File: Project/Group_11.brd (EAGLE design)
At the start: 29 parts, among them J1 POWER_JACKPTH_LOCK, U1 +12v

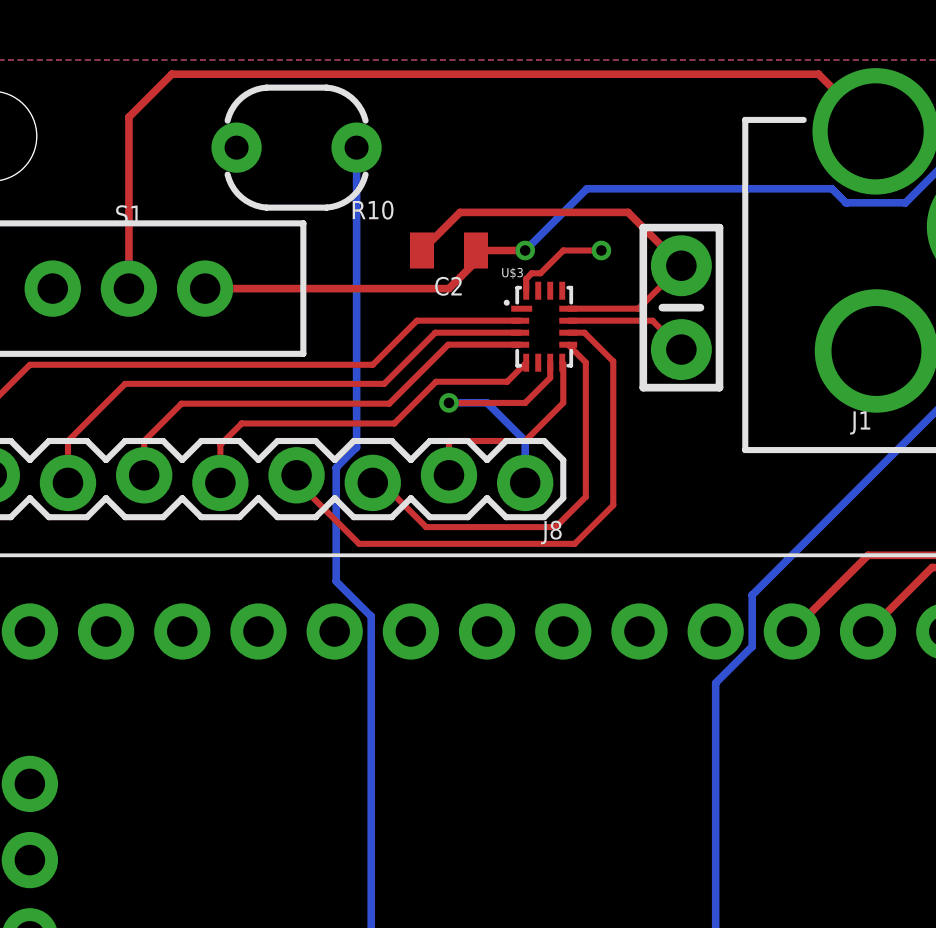
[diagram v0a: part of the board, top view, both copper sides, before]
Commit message: Aggiunta collegamenti board
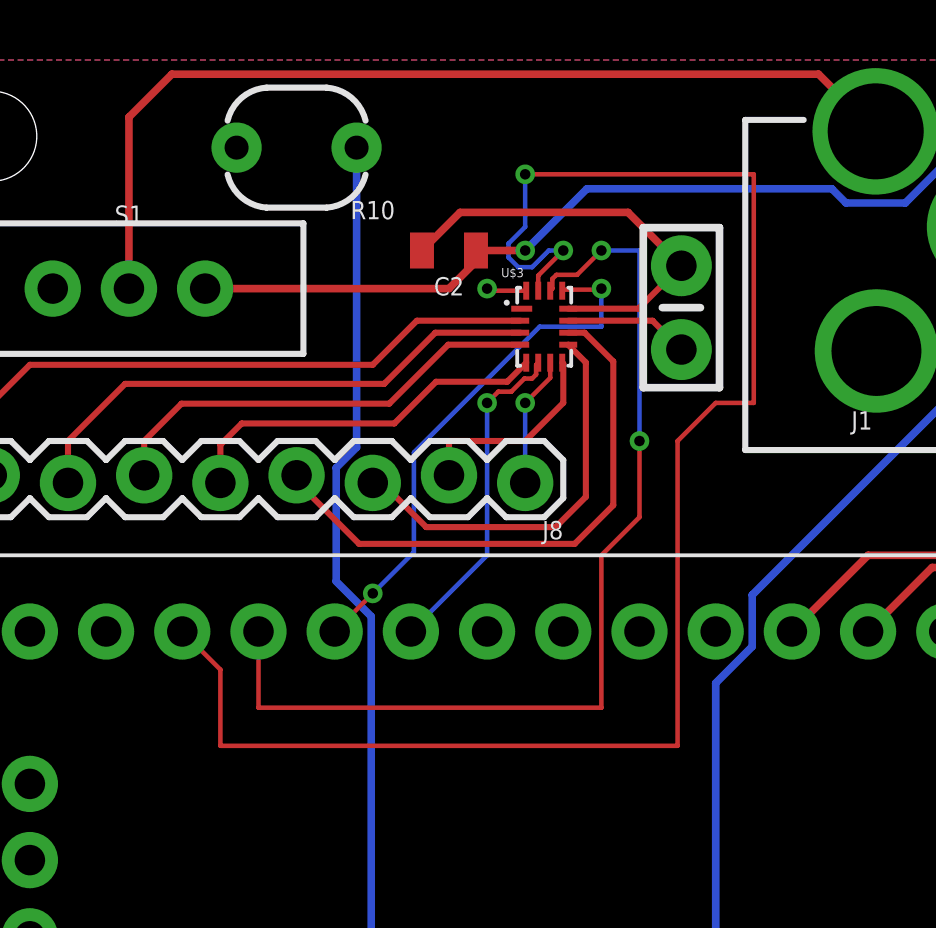
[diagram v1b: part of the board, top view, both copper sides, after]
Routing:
- net MUX_A0: track 0.00 -> 54.9 mm, vias 0 -> 2
- net MUX_A1: track 0.00 -> 33.5 mm, vias 0 -> 2
- net MUX_A2: track 0.00 -> 17.7 mm, vias 0 -> 2
- net MUX_OUT: track 0.00 -> 11.1 mm, vias 0 -> 1
- net N$11: track 8.69 -> 4.35 mm
- net 5V: track 46.6 -> 44.7 mm
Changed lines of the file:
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@@
 <wire x1="21.755" y1="38.3" x2="24.56501875" y2="38.3" width="0.2032" layer="1"/>
 <wire x1="24.56501875" y1="38.3" x2="25.527" y2="37.338" width="0.2032" layer="1"/>
-<wire x1="20.53926875" y1="39.8794" x2="20.8294" y2="39.8794" width="0.2032" layer="1"/>
-<wire x1="20.8294" y1="39.8794" x2="21.59" y2="40.64" width="0.2032" layer="1"/>
-<wire x1="21.59" y1="40.64" x2="22.86" y2="40.64" width="0.2032" layer="1"/>
-<via x="22.86" y="40.64" extent="1-16" drill="0.35"/>
+<via x="19.05" y="39.37" extent="1-16" drill="0.35"/>
 <wire x1="41.314" y1="33.147" x2="41.06" y2="32.893" width="0.254" layer="1"/>
 <wire x1="41.06" y1="32.893" x2="38.1" y2="32.893" width="0.254" layer="1"/>
@@
 <vertex x="0.508" y="1.27"/>
 </polygon>
-<wire x1="20.355" y1="39.3" x2="20.355" y2="39.69513125" width="0.2032" layer="1"/>
-<wire x1="20.355" y1="39.69513125" x2="20.53926875" y2="39.8794" width="0.2032" layer="1"/>
 <wire x1="41.91" y1="34.837" x2="40.386" y2="36.361" width="0.254" layer="1"/>
 <wire x1="40.386" y1="36.361" x2="40.386" y2="38.139" width="0.254" layer="1"/>
 <wire x1="41.314" y1="33.147" x2="41.314" y2="34.241" width="0.254" layer="1"/>
 <wire x1="41.314" y1="34.241" x2="41.91" y2="34.837" width="0.254" layer="1"/>
+<wire x1="20.355" y1="39.3" x2="19.12" y2="39.3" width="0.1524" layer="1"/>
+<wire x1="19.12" y1="39.3" x2="19.05" y2="39.37" width="0.1524" layer="1"/>
 </signal>
 <signal name="N$9">
@@
 <contactref element="J8" pad="1"/>
 <contactref element="U$3" pad="7"/>
-<wire x1="20.32" y1="35.56" x2="17.78" y2="35.56" width="0.2032" layer="1"/>
-<via x="17.78" y="35.56" extent="1-16" drill="0.35"/>
-<wire x1="17.78" y1="35.56" x2="19.05" y2="35.56" width="0.254" layer="16"/>
-<wire x1="19.05" y1="35.56" x2="20.32" y2="34.29" width="0.254" layer="16"/>
-<wire x1="20.32" y1="34.29" x2="20.32" y2="32.893" width="0.254" layer="16"/>
-<wire x1="21.155" y1="36.9" x2="21.155" y2="36.395" width="0.2032" layer="1"/>
-<wire x1="21.155" y1="36.395" x2="20.32" y2="35.56" width="0.2032" layer="1"/>
+<wire x1="20.32" y1="32.893" x2="20.32" y2="35.56" width="0.1524" layer="16"/>
+<via x="20.32" y="35.56" extent="1-16" drill="0.35"/>
+<wire x1="20.32" y1="35.56" x2="21.155" y2="36.395" width="0.1524" layer="1"/>
+<wire x1="21.155" y1="36.395" x2="21.155" y2="36.9" width="0.1524" layer="1"/>
 </signal>
 <signal name="N$12">
@@
 <contactref element="U$3" pad="6"/>
 <contactref element="U$2" pad="21"/>
-<wire x1="16.51" y1="27.94" x2="20.755" y2="36.9" width="0" layer="19" extent="1-1"/>
+<wire x1="16.51" y1="27.94" x2="19.05" y2="30.48" width="0.1524" layer="16"/>
+<wire x1="19.05" y1="30.48" x2="19.05" y2="35.56" width="0.1524" layer="16"/>
+<via x="19.05" y="35.56" extent="1-16" drill="0.35"/>
+<wire x1="19.05" y1="35.56" x2="19.4248" y2="35.9348" width="0.1524" layer="1"/>
+<wire x1="19.4248" y1="35.9348" x2="19.856775" y2="35.9348" width="0.1524" layer="1"/>
+<wire x1="20.293375" y1="36.3714" x2="20.5496875" y2="36.3714" width="0.1524" layer="1"/>
+<wire x1="19.856775" y1="35.9348" x2="20.293375" y2="36.3714" width="0.1524" layer="1"/>
+<wire x1="20.6852" y1="36.8302" x2="20.755" y2="36.9" width="0.1524" layer="1"/>
+<wire x1="20.5496875" y1="36.3714" x2="20.6852" y2="36.5069125" width="0.1524" layer="1"/>
+<wire x1="20.6852" y1="36.5069125" x2="20.6852" y2="36.8302" width="0.1524" layer="1"/>
 </signal>
 <signal name="MUX_A0">
 <contactref element="U$3" pad="15"/>
 <contactref element="U$2" pad="24"/>
-<wire x1="8.89" y1="27.94" x2="20.755" y2="39.3" width="0" layer="19" extent="1-1"/>
+<wire x1="8.89" y1="27.94" x2="10.16" y2="26.67" width="0.1524" layer="1"/>
+<wire x1="10.16" y1="26.67" x2="10.16" y2="24.13" width="0.1524" layer="1"/>
+<wire x1="10.16" y1="24.13" x2="25.4" y2="24.13" width="0.1524" layer="1"/>
+<wire x1="25.4" y1="24.13" x2="25.4" y2="34.29" width="0.1524" layer="1"/>
+<wire x1="25.4" y1="34.29" x2="26.67" y2="35.56" width="0.1524" layer="1"/>
+<wire x1="26.67" y1="35.56" x2="27.94" y2="35.56" width="0.1524" layer="1"/>
+<wire x1="27.94" y1="35.56" x2="27.94" y2="43.18" width="0.1524" layer="1"/>
+<wire x1="27.94" y1="43.18" x2="20.32" y2="43.18" width="0.1524" layer="1"/>
+<via x="20.32" y="43.18" extent="1-16" drill="0.35"/>
+<wire x1="19.764" y1="40.87030625" x2="19.764" y2="40.40969375" width="0.1524" layer="16"/>
+<wire x1="19.764" y1="40.40969375" x2="20.08969375" y2="40.084" width="0.1524" layer="16"/>
+<wire x1="20.08969375" y1="40.084" x2="20.55030625" y2="40.084" width="0.1524" layer="16"/>
+<wire x1="20.32" y1="43.18" x2="20.32" y2="41.42630625" width="0.1524" layer="16"/>
+<wire x1="20.32" y1="41.42630625" x2="19.764" y2="40.87030625" width="0.1524" layer="16"/>
+<wire x1="20.55030625" y1="40.084" x2="21.10630625" y2="40.64" width="0.1524" layer="16"/>
+<wire x1="21.10630625" y1="40.64" x2="21.59" y2="40.64" width="0.1524" layer="16"/>
+<via x="21.59" y="40.64" extent="1-16" drill="0.35"/>
+<wire x1="21.59" y1="40.64" x2="20.755" y2="39.805" width="0.1524" layer="1"/>
+<wire x1="20.755" y1="39.805" x2="20.755" y2="39.3" width="0.1524" layer="1"/>
 </signal>
 <signal name="MUX_A1">
 <contactref element="U$3" pad="14"/>
 <contactref element="U$2" pad="23"/>
-<wire x1="11.43" y1="27.94" x2="21.155" y2="39.3" width="0" layer="19" extent="1-1"/>
+<wire x1="11.43" y1="27.94" x2="11.43" y2="25.4" width="0.1524" layer="1"/>
+<wire x1="11.43" y1="25.4" x2="22.86" y2="25.4" width="0.1524" layer="1"/>
+<wire x1="22.86" y1="25.4" x2="22.86" y2="30.48" width="0.1524" layer="1"/>
+<wire x1="22.86" y1="30.48" x2="24.13" y2="31.75" width="0.1524" layer="1"/>
+<wire x1="24.13" y1="31.75" x2="24.13" y2="34.29" width="0.1524" layer="1"/>
+<via x="24.13" y="34.29" extent="1-16" drill="0.35"/>
+<wire x1="24.13" y1="34.29" x2="24.13" y2="40.64" width="0.1524" layer="16"/>
+<wire x1="24.13" y1="40.64" x2="22.86" y2="40.64" width="0.1524" layer="16"/>
+<via x="22.86" y="40.64" extent="1-16" drill="0.35"/>
+<wire x1="21.3603125" y1="39.8286" x2="21.2264" y2="39.6946875" width="0.1524" layer="1"/>
+<wire x1="22.86" y1="40.64" x2="22.0486" y2="39.8286" width="0.1524" layer="1"/>
+<wire x1="21.2264" y1="39.6946875" x2="21.2264" y2="39.3714" width="0.1524" layer="1"/>
+<wire x1="21.2264" y1="39.3714" x2="21.155" y2="39.3" width="0.1524" layer="1"/>
+<wire x1="22.0486" y1="39.8286" x2="21.3603125" y2="39.8286" width="0.1524" layer="1"/>
 </signal>
 <signal name="MUX_A2">
 <contactref element="U$3" pad="13"/>
 <contactref element="U$2" pad="22"/>
-<wire x1="13.97" y1="27.94" x2="21.555" y2="39.3" width="0" layer="19" extent="1-1"/>
+<wire x1="13.97" y1="27.94" x2="15.24" y2="29.21" width="0.1524" layer="1"/>
+<via x="15.24" y="29.21" extent="1-16" drill="0.35"/>
+<wire x1="15.24" y1="29.21" x2="16.6116" y2="30.5816" width="0.1524" layer="16"/>
+<wire x1="16.6116" y1="30.5816" x2="16.6116" y2="33.90790625" width="0.1524" layer="16"/>
+<wire x1="21.555" y1="39.335" x2="21.555" y2="39.3" width="0.1524" layer="1"/>
+<wire x1="16.6116" y1="33.90790625" x2="20.80369375" y2="38.1" width="0.1524" layer="16"/>
+<wire x1="20.80369375" y1="38.1" x2="22.86" y2="38.1" width="0.1524" layer="16"/>
+<wire x1="22.86" y1="38.1" x2="22.86" y2="39.37" width="0.1524" layer="16"/>
+<via x="22.86" y="39.37" extent="1-16" drill="0.35"/>
+<wire x1="22.86" y1="39.37" x2="22.825" y2="39.335" width="0.1524" layer="1"/>
+<wire x1="22.825" y1="39.335" x2="21.555" y2="39.335" width="0.1524" layer="1"/>
 </signal>
 </signals>

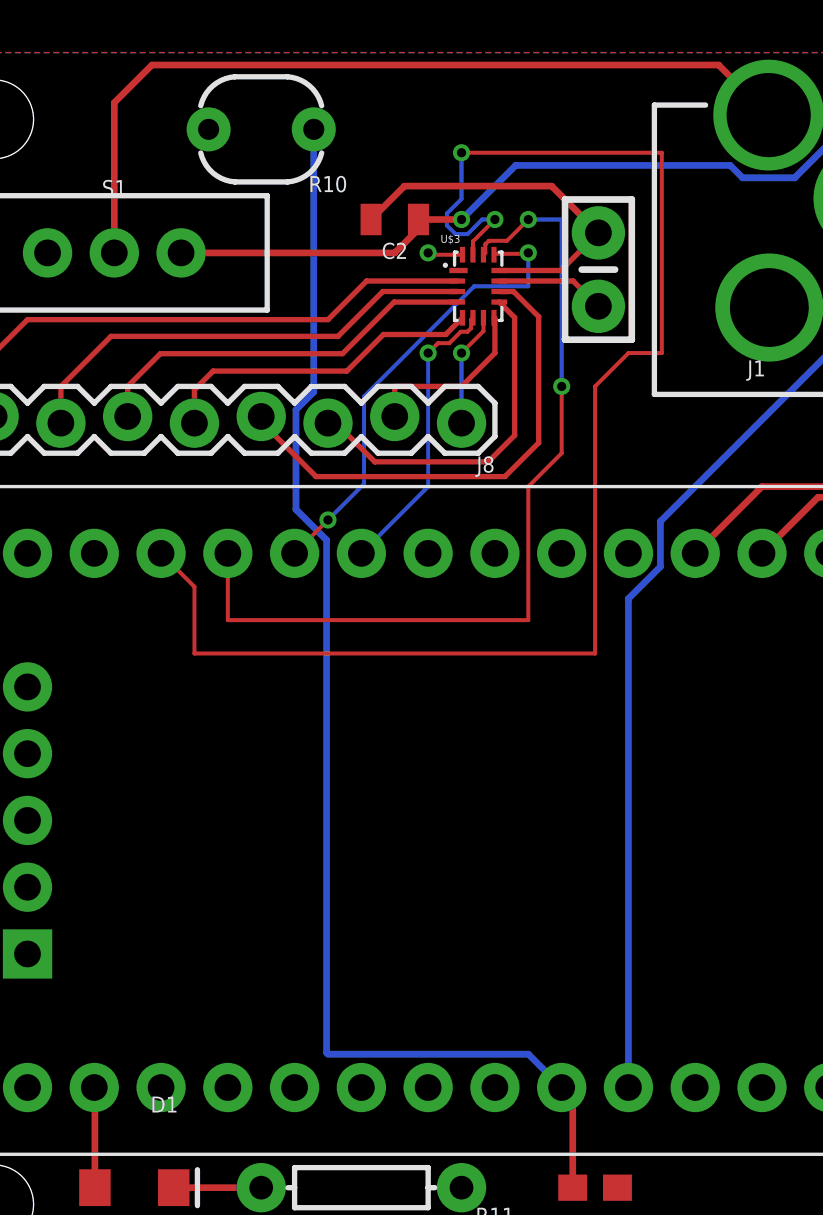
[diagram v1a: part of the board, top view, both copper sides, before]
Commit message: Correzione clearance
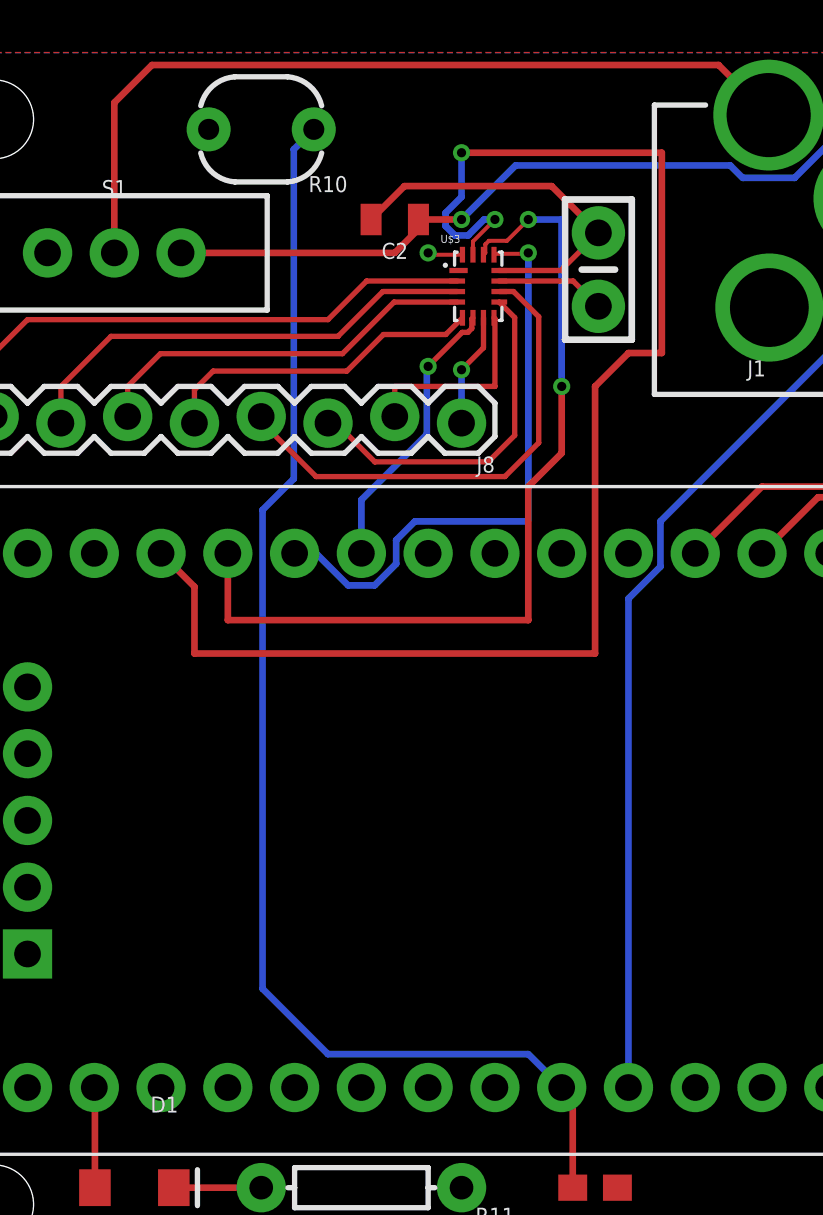
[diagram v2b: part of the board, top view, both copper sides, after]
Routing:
- net MUX_A2: track 17.7 -> 22.5 mm, vias 2 -> 1
- net PHOTO_OUT: track 49.4 -> 50.4 mm
- net N$12: track 6.83 -> 7.58 mm
